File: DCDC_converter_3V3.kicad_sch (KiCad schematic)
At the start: 24 parts, among them J6 DC barrel assy, J8 Dell DC jack, U1 LMR380x0

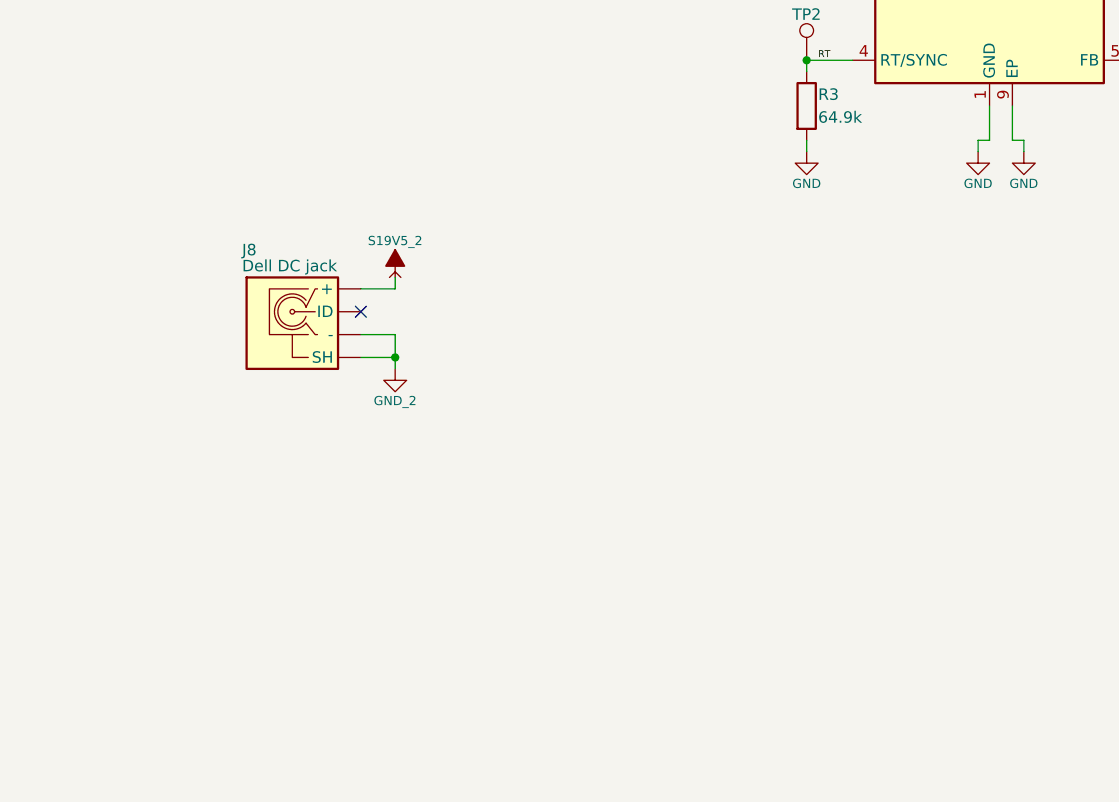
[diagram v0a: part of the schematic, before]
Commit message: reorganised sch and pcb
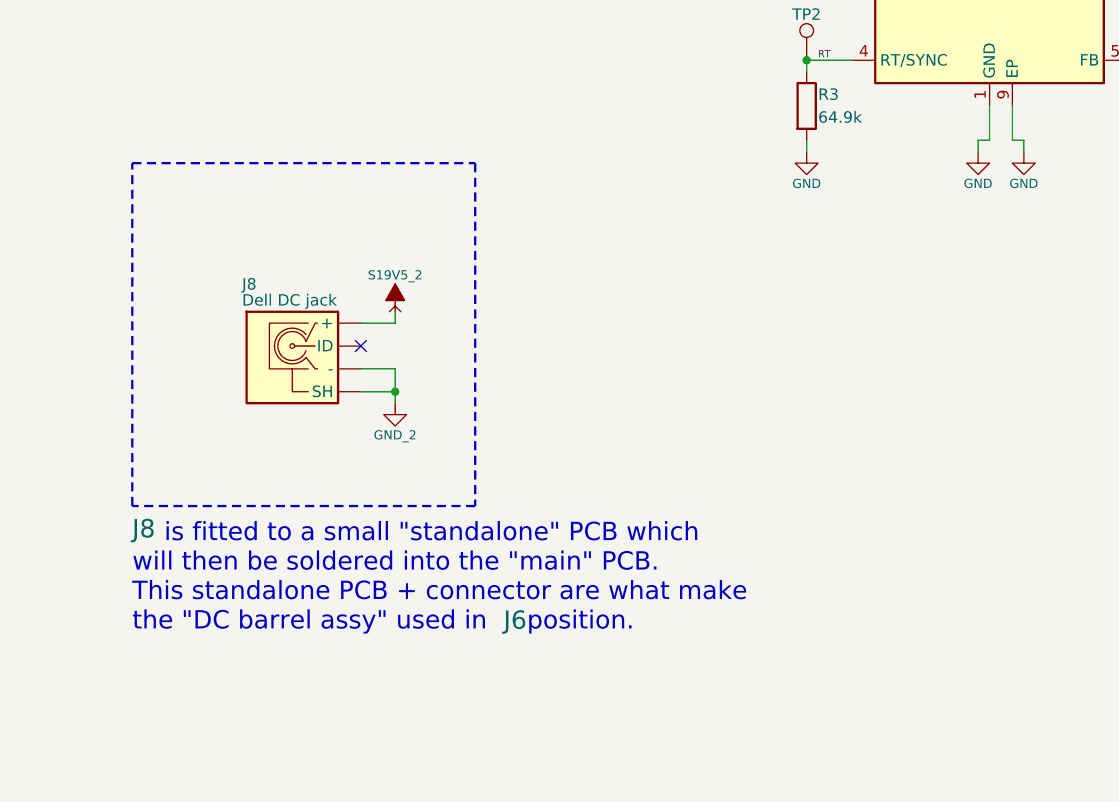
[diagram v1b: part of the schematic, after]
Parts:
- J6: Assy (none) -> ${REFERENCE}
- J8: BarrelConn (none) -> ${REFERENCE}
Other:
- note added: "is fitted to a small "standalone" PCB which will then be soldered into the "main" PCB. This standalone PCB + connector are what make the "DC barrel assy" used in position."
- moved on the sheet: J8
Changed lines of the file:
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@@
 	(paper "A4")
 	(rectangle
+		(start 25.4 114.3)
+		(end 63.5 152.4)
+		(stroke
+			(width 0.254)
+			(type dash)
+			(color 0 0 0 1)
+		)
+		(fill
+			(type none)
+		)
+	)
+	(rectangle
 		(start 13.97 13.97)
 		(end 48.26 31.75)
@@
 		)
 	)
+	(text "    is fitted to a small \"standalone\" PCB which\nwill then be soldered into the \"main\" PCB.\nThis standalone PCB + connector are what make\nthe \"DC barrel assy\" used in     position."
+		(exclude_from_sim no)
+		(at 25.4 154.305 0)
+		(effects
+			(font
+				(size 2.032 2.032)
+				(color 0 0 0 1)
+			)
+			(justify left top)
+		)
+	)
 	(text "Return to front sheet"
 		(exclude_from_sim no)
@@
 	)
 	(junction
-		(at 54.61 135.89)
+		(at 54.61 139.7)
 		(diameter 0)
 		(color 0 0 0 0)
@@
 	)
 	(no_connect
-		(at 50.8 130.81)
+		(at 50.8 134.62)
 	)
 	(wire
@@
 	(wire
 		(pts
-			(xy 50.8 133.35) (xy 54.61 133.35)
+			(xy 50.8 137.16) (xy 54.61 137.16)
 		)
 		(stroke
@@
 	(wire
 		(pts
-			(xy 54.61 133.35) (xy 54.61 135.89)
+			(xy 54.61 137.16) (xy 54.61 139.7)
 		)
 		(stroke
@@
 	(wire
 		(pts
-			(xy 54.61 135.89) (xy 54.61 137.16)
+			(xy 54.61 139.7) (xy 54.61 140.97)
 		)
 		(stroke
@@
 	(wire
 		(pts
-			(xy 54.61 128.27) (xy 54.61 127)
+			(xy 54.61 132.08) (xy 54.61 130.81)
 		)
 		(stroke
@@
 	(wire
 		(pts
-			(xy 50.8 128.27) (xy 54.61 128.27)
+			(xy 50.8 132.08) (xy 54.61 132.08)
 		)
 		(stroke
@@
 	(wire
 		(pts
-			(xy 50.8 135.89) (xy 54.61 135.89)
+			(xy 50.8 139.7) (xy 54.61 139.7)
 		)
 		(stroke
@@
 	(symbol
 		(lib_id "personal:Cosmetic_PWR_SRC")
-		(at 54.61 127 0)
+		(at 54.61 130.81 0)
 		(unit 1)
 		(body_style 1)
@@
 		(fields_autoplaced yes)
 		(property "Reference" "Pwr014"
-			(at 54.61 122.682 0)
+			(at 54.61 126.492 0)
 			(hide yes)
 			(show_name no)
@@
 		)
 		(property "Value" "S19V5_2"
-			(at 54.61 122.936 0)
+			(at 54.61 126.746 0)
 			(show_name no)
 			(do_not_autoplace yes)
@@
 		)
 		(property "Footprint" ""
-			(at 54.61 127 0)
+			(at 54.61 130.81 0)
 			(hide yes)
 			(show_name no)
@@
 		)
 		(property "Datasheet" ""
-			(at 54.61 127 0)
+			(at 54.61 130.81 0)
 			(hide yes)
 			(show_name no)
@@
 		)
 		(property "Description" "Local power symbol (source), cosmetic use only"
-			(at 54.61 127 0)
+			(at 54.61 130.81 0)
 			(hide yes)
 			(show_name no)
@@
 	(symbol
 		(lib_id "personal:Cosmetic_GND")
-		(at 54.61 137.16 0)
+		(at 54.61 140.97 0)
 		(unit 1)
 		(body_style 1)
@@
 		(fields_autoplaced yes)
 		(property "Reference" "Pwr017"
-			(at 54.61 132.842 0)
+			(at 54.61 136.652 0)
 			(hide yes)
 			(show_name no)
@@
 		)
 		(property "Value" "GND_2"
-			(at 54.61 140.716 0)
+			(at 54.61 144.526 0)
 			(show_name no)
 			(do_not_autoplace yes)
@@
 		)
 		(property "Footprint" ""
-			(at 54.61 137.16 0)
+			(at 54.61 140.97 0)
 			(hide yes)
 			(show_name no)
@@
 		)
 		(property "Datasheet" ""
-			(at 54.61 137.16 0)
+			(at 54.61 140.97 0)
 			(hide yes)
 			(show_name no)
@@
 		)
 		(property "Description" "Local power symbol (sink), cosmetic use only"
-			(at 54.61 137.16 0)
+			(at 54.61 140.97 0)
 			(hide yes)
 			(show_name no)
@@
 		(in_pos_files yes)
 		(dnp no)
-		(fields_autoplaced yes)
 		(property "Reference" "J6"
 			(at 36.322 70.612 0)
@@
 			)
 		)
+		(property "Assy" "${REFERENCE}"
+			(at 67.945 165.1 0)
+			(show_name no)
+			(do_not_autoplace no)
+			(effects
+				(font
+					(size 2.032 2.032)
+				)
+			)
+		)
 		(pin "2"
 		)
@@
 	(symbol
 		(lib_id "personal:Dell_DC_barrel_jack")
-		(at 43.18 132.08 0)
+		(at 43.18 135.89 0)
 		(unit 1)
 		(body_style 1)
@@
 		(in_pos_files yes)
 		(dnp no)
-		(fields_autoplaced yes)
 		(property "Reference" "J8"
-			(at 37.592 123.952 0)
+			(at 37.592 127.762 0)
 			(show_name no)
 			(do_not_autoplace yes)
@@
 		)
 		(property "Value" "Dell DC jack"
-			(at 37.592 125.73 0)
+			(at 37.592 129.54 0)
 			(show_name no)
 			(do_not_autoplace yes)
@@
 		)
 		(property "Footprint" "Personal:Dell DC jack"
-			(at 43.18 132.08 0)
+			(at 43.18 135.89 0)
 			(hide yes)
 			(show_name no)
@@
 		)
 		(property "Datasheet" ""
-			(at 43.18 132.08 0)
+			(at 43.18 135.89 0)
 			(hide yes)
 			(show_name no)
@@
 		)
 		(property "Description" ""
-			(at 43.18 132.08 0)
+			(at 43.18 135.89 0)
 			(hide yes)
 			(show_name no)
@@
 				)
 			)
+		)
+		(property "BarrelConn" "${REFERENCE}"
+			(at 26.67 154.94 0)
+			(show_name no)
+			(do_not_autoplace no)
+			(effects
+				(font
+					(size 2.032 2.032)
+				)
+			)
